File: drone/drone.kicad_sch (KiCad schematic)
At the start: 46 parts, among them J2 HMC5883, J3 Conn_01x03_Pin, U2 MPU-6050, U3 MP2303ADN

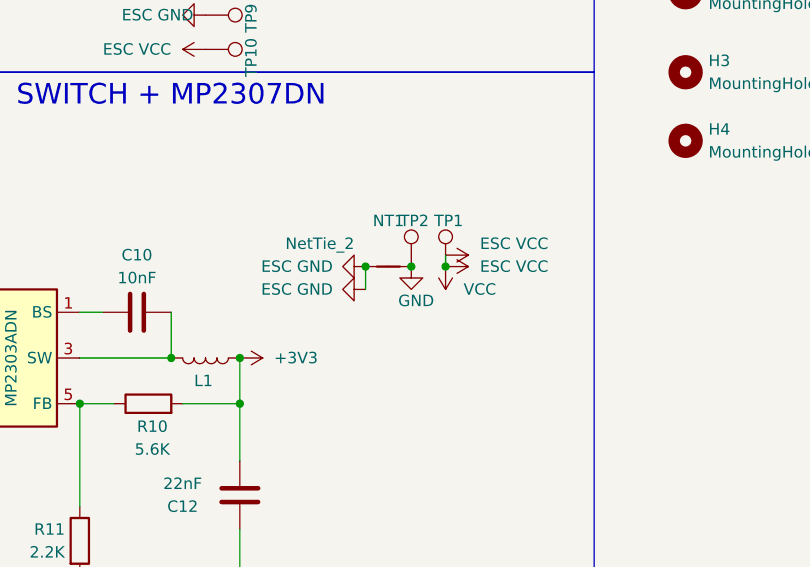
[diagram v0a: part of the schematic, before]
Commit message: ho
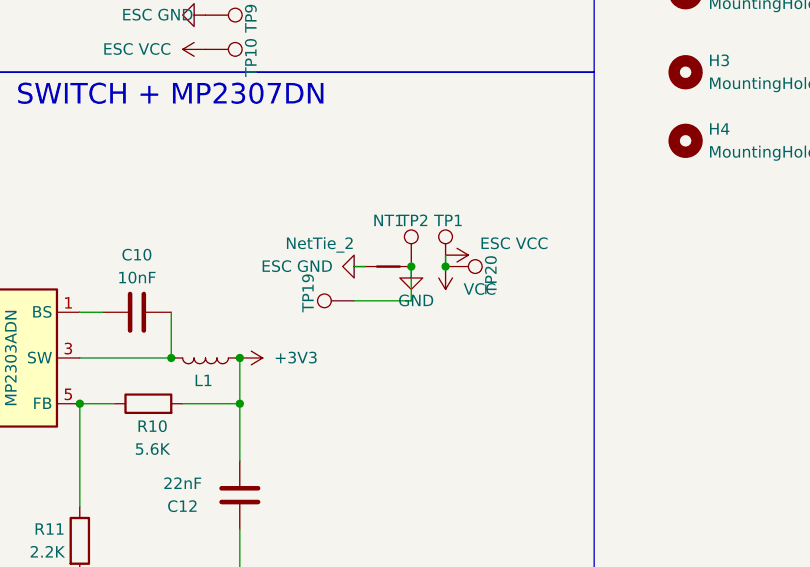
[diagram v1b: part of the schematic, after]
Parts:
- added TP19, TP20: TestPoint, TestPoint:TestPoint_Pad_2.5x2.5mm, symbol Connector:TestPoint
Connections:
- net ESC VCC: now also TP20.1
- net GND: now also TP19.1
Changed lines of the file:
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@@
 	)
 	(junction
-		(at 151.13 157.48)
-		(diameter 0)
-		(color 0 0 0 0)
-	)
-	(junction
 		(at 224.79 38.1)
 		(diameter 0)
@@
 	(wire
 		(pts
+			(xy 149.86 157.48) (xy 151.13 157.48)
+		)
+		(stroke
+			(width 0)
+			(type default)
+		)
+	)
+	(wire
+		(pts
 			(xy 95.25 66.04) (xy 91.44 66.04)
 		)
@@
 	(wire
 		(pts
+			(xy 156.21 161.29) (xy 156.21 157.48)
+		)
+		(stroke
+			(width 0)
+			(type default)
+		)
+	)
+	(wire
+		(pts
 			(xy 231.14 40.64) (xy 224.79 40.64)
 		)
@@
 	(wire
 		(pts
-			(xy 234.95 66.04) (xy 234.95 80.01)
+			(xy 149.86 161.29) (xy 156.21 161.29)
 		)
 		(stroke
@@
 	(wire
 		(pts
-			(xy 100.33 73.66) (xy 91.44 73.66)
+			(xy 234.95 66.04) (xy 234.95 80.01)
 		)
 		(stroke
@@
 	(wire
 		(pts
-			(xy 223.52 80.01) (xy 223.52 77.47)
+			(xy 100.33 73.66) (xy 91.44 73.66)
 		)
 		(stroke
@@
 	(wire
 		(pts
-			(xy 91.44 66.04) (xy 87.63 66.04)
+			(xy 223.52 80.01) (xy 223.52 77.47)
 		)
 		(stroke
@@
 	(wire
 		(pts
-			(xy 119.38 172.72) (xy 123.19 172.72)
+			(xy 91.44 66.04) (xy 87.63 66.04)
 		)
 		(stroke
@@
 	(wire
 		(pts
-			(xy 151.13 157.48) (xy 151.13 160.02)
+			(xy 119.38 172.72) (xy 123.19 172.72)
 		)
 		(stroke
@@
 	)
 	(symbol
-		(lib_id "power:GND")
-		(at 151.13 160.02 270)
-		(unit 1)
-		(body_style 1)
-		(exclude_from_sim no)
-		(in_bom yes)
-		(on_board yes)
-		(in_pos_files yes)
-		(dnp no)
-		(property "Reference" "#PWR044"
-			(at 144.78 160.02 0)
-			(hide yes)
-			(show_name no)
-			(do_not_autoplace no)
-			(effects
-				(font
-					(size 1.27 1.27)
-				)
-			)
-		)
-		(property "Value" "ESC GND"
-			(at 143.51 160.02 90)
-			(show_name no)
-			(do_not_autoplace no)
-			(effects
-				(font
-					(size 1.27 1.27)
-				)
-			)
-		)
-		(property "Footprint" ""
-			(at 151.13 160.02 0)
-			(hide yes)
-			(show_name no)
-			(do_not_autoplace no)
-			(effects
-				(font
-					(size 1.27 1.27)
-				)
-			)
-		)
-		(property "Datasheet" ""
-			(at 151.13 160.02 0)
-			(hide yes)
-			(show_name no)
-			(do_not_autoplace no)
-			(effects
-				(font
-					(size 1.27 1.27)
-				)
-			)
-		)
-		(property "Description" "Power symbol creates a global label with name \"GND\" , ground"
-			(at 151.13 160.02 0)
-			(hide yes)
-			(show_name no)
-			(do_not_autoplace no)
-			(effects
-				(font
-					(size 1.27 1.27)
-				)
-			)
-		)
-		(pin "1"
-		)
-		(instances
-			(project "drone"
-				(path "/fa7edb3b-7a08-4951-b563-6ccff1e89ead"
-					(reference "#PWR044")
-					(unit 1)
-				)
-			)
-		)
-	)
-	(symbol
 		(lib_id "power:VCC")
 		(at 30.48 161.29 90)
@@
 	)
 	(symbol
+		(lib_id "Connector:TestPoint")
+		(at 149.86 161.29 90)
+		(unit 1)
+		(body_style 1)
+		(exclude_from_sim no)
+		(in_bom yes)
+		(on_board yes)
+		(in_pos_files yes)
+		(dnp no)
+		(property "Reference" "TP19"
+			(at 144.78 162.56 0)
+			(show_name no)
+			(do_not_autoplace no)
+			(effects
+				(font
+					(size 1.27 1.27)
+				)
+				(justify left)
+			)
+		)
+		(property "Value" "TestPoint"
+			(at 147.8279 158.75 0)
+			(hide yes)
+			(show_name no)
+			(do_not_autoplace no)
+			(effects
+				(font
+					(size 1.27 1.27)
+				)
+				(justify left)
+			)
+		)
+		(property "Footprint" "TestPoint:TestPoint_Pad_2.5x2.5mm"
+			(at 149.86 156.21 0)
+			(hide yes)
+			(show_name no)
+			(do_not_autoplace no)
+			(effects
+				(font
+					(size 1.27 1.27)
+				)
+			)
+		)
+		(property "Datasheet" ""
+			(at 149.86 156.21 0)
+			(hide yes)
+			(show_name no)
+			(do_not_autoplace no)
+			(effects
+				(font
+					(size 1.27 1.27)
+				)
+			)
+		)
+		(property "Description" "test point"
+			(at 149.86 161.29 0)
+			(hide yes)
+			(show_name no)
+			(do_not_autoplace no)
+			(effects
+				(font
+					(size 1.27 1.27)
+				)
+			)
+		)
+		(pin "1"
+		)
+		(instances
+			(project "drone"
+				(path "/fa7edb3b-7a08-4951-b563-6ccff1e89ead"
+					(reference "TP19")
+					(unit 1)
+				)
+			)
+		)
+	)
+	(symbol
 		(lib_id "Device:C")
 		(at 99.06 182.88 0)
@@
 	)
 	(symbol
-		(lib_id "power:VCC")
-		(at 160.02 157.48 270)
-		(unit 1)
-		(body_style 1)
-		(exclude_from_sim no)
-		(in_bom yes)
-		(on_board yes)
-		(in_pos_files yes)
-		(dnp no)
-		(property "Reference" "#PWR043"
-			(at 156.21 157.48 0)
-			(hide yes)
-			(show_name no)
-			(do_not_autoplace no)
-			(effects
-				(font
-					(size 1.27 1.27)
-				)
-			)
-		)
-		(property "Value" "ESC VCC"
-			(at 167.64 157.48 90)
-			(show_name no)
-			(do_not_autoplace no)
-			(effects
-				(font
-					(size 1.27 1.27)
-				)
-			)
-		)
-		(property "Footprint" ""
-			(at 160.02 157.48 0)
-			(hide yes)
-			(show_name no)
-			(do_not_autoplace no)
-			(effects
-				(font
-					(size 1.27 1.27)
-				)
-			)
-		)
-		(property "Datasheet" ""
-			(at 160.02 157.48 0)
-			(hide yes)
-			(show_name no)
-			(do_not_autoplace no)
-			(effects
-				(font
-					(size 1.27 1.27)
-				)
-			)
-		)
-		(property "Description" "Power symbol creates a global label with name \"VCC\""
-			(at 160.02 157.48 0)
-			(hide yes)
-			(show_name no)
-			(do_not_autoplace no)
-			(effects
-				(font
-					(size 1.27 1.27)
-				)
-			)
-		)
-		(pin "1"
-		)
-		(instances
-			(project "drone"
-				(path "/fa7edb3b-7a08-4951-b563-6ccff1e89ead"
-					(reference "#PWR043")
-					(unit 1)
-				)
-			)
-		)
-	)
-	(symbol
 		(lib_id "Connector:TestPoint")
 		(at 160.02 157.48 0)
@@
 					(unit 1)
 				)
+			)
+		)
+	)
+	(symbol
+		(lib_id "Connector:TestPoint")
+		(at 160.02 157.48 270)
+		(unit 1)
+		(body_style 1)
+		(exclude_from_sim no)
+		(in_bom yes)
+		(on_board yes)
+		(in_pos_files yes)
+		(dnp no)
+		(property "Reference" "TP20"
+			(at 165.1 156.21 0)
+			(show_name no)
+			(do_not_autoplace no)
+			(effects
+				(font
+					(size 1.27 1.27)
+				)
+				(justify left)
+			)
+		)
+		(property "Value" "TestPoint"
+			(at 162.0521 160.02 0)
+			(hide yes)
+			(show_name no)
+			(do_not_autoplace no)
+			(effects
+				(font
+					(size 1.27 1.27)
+				)
+				(justify left)
+			)
+		)
+		(property "Footprint" "TestPoint:TestPoint_Pad_2.5x2.5mm"
+			(at 160.02 162.56 0)
+			(hide yes)
+			(show_name no)
+			(do_not_autoplace no)
+			(effects
+				(font
+					(size 1.27 1.27)
+				)
+			)
+		)
+		(property "Datasheet" ""
+			(at 160.02 162.56 0)
+			(hide yes)
+			(show_name no)
+			(do_not_autoplace no)
+			(effects
+				(font
+					(size 1.27 1.27)
+				)
+			)
+		)
+		(property "Description" "test point"
+			(at 160.02 157.48 0)
+			(hide yes)
+			(show_name no)
+			(do_not_autoplace no)
+			(effects
+				(font
+					(size 1.27 1.27)
+				)
+			)
+		)
+		(pin "1"
+		)
+		(instances
+			(project "drone"
+				(path "/fa7edb3b-7a08-4951-b563-6ccff1e89ead"
+					(reference "TP20")
+					(unit 1)
+				)
